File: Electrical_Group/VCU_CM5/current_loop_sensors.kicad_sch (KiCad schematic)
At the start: 16 parts, among them J11 Conn_01x30_Socket

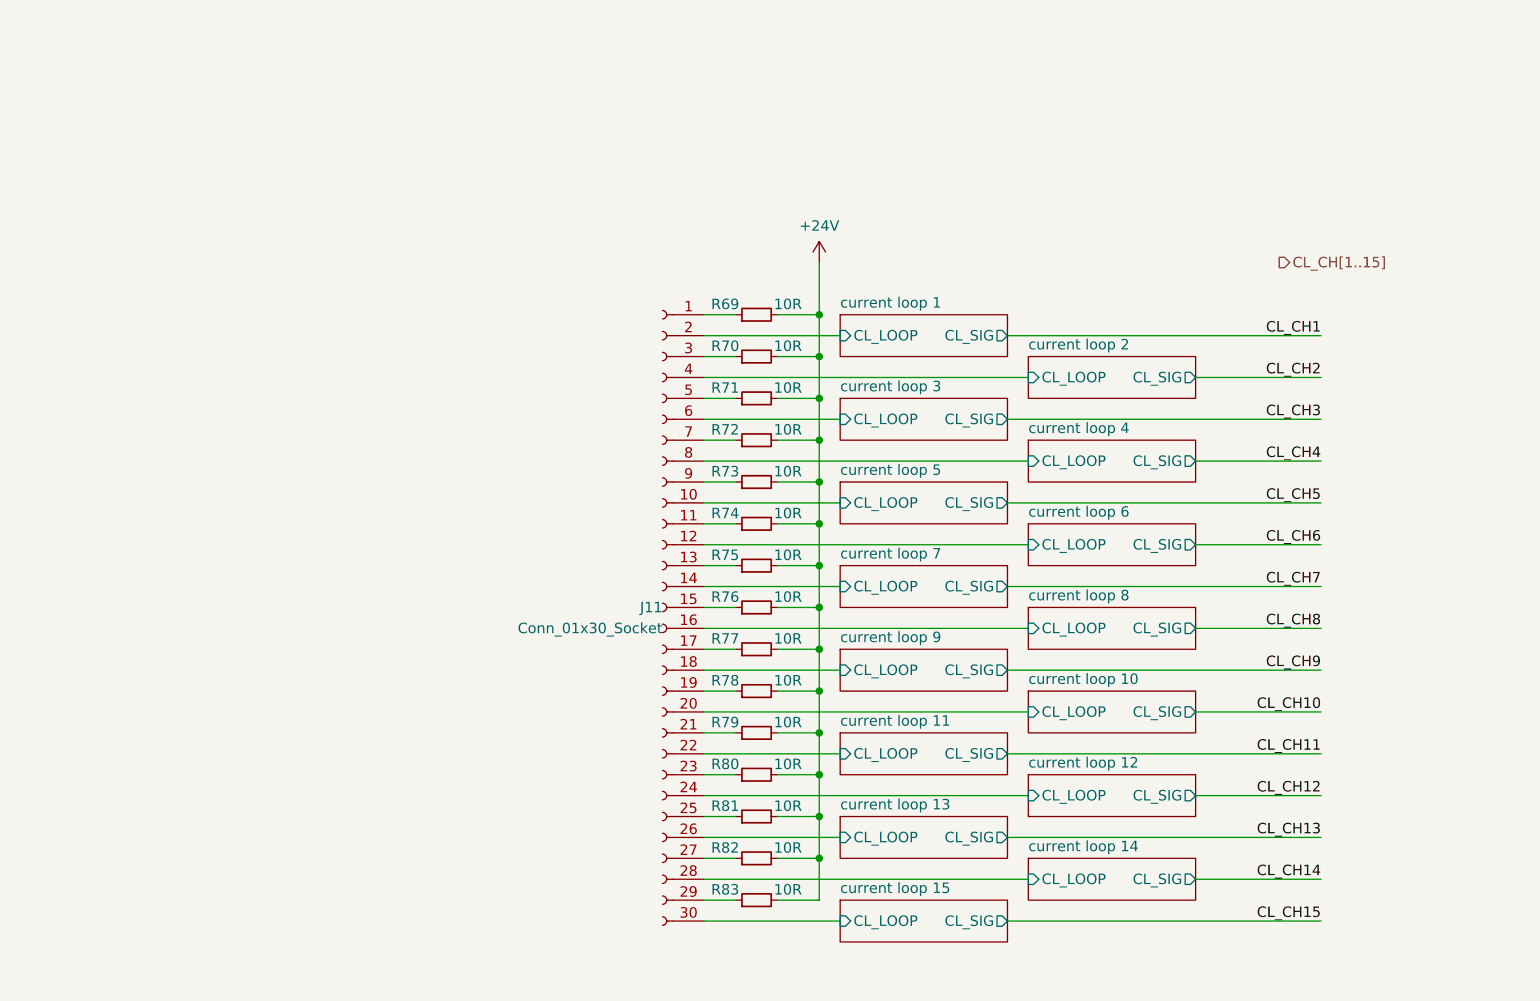
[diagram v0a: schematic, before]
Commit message: [VCU_CM5] update to V1.0
still needs many modifications
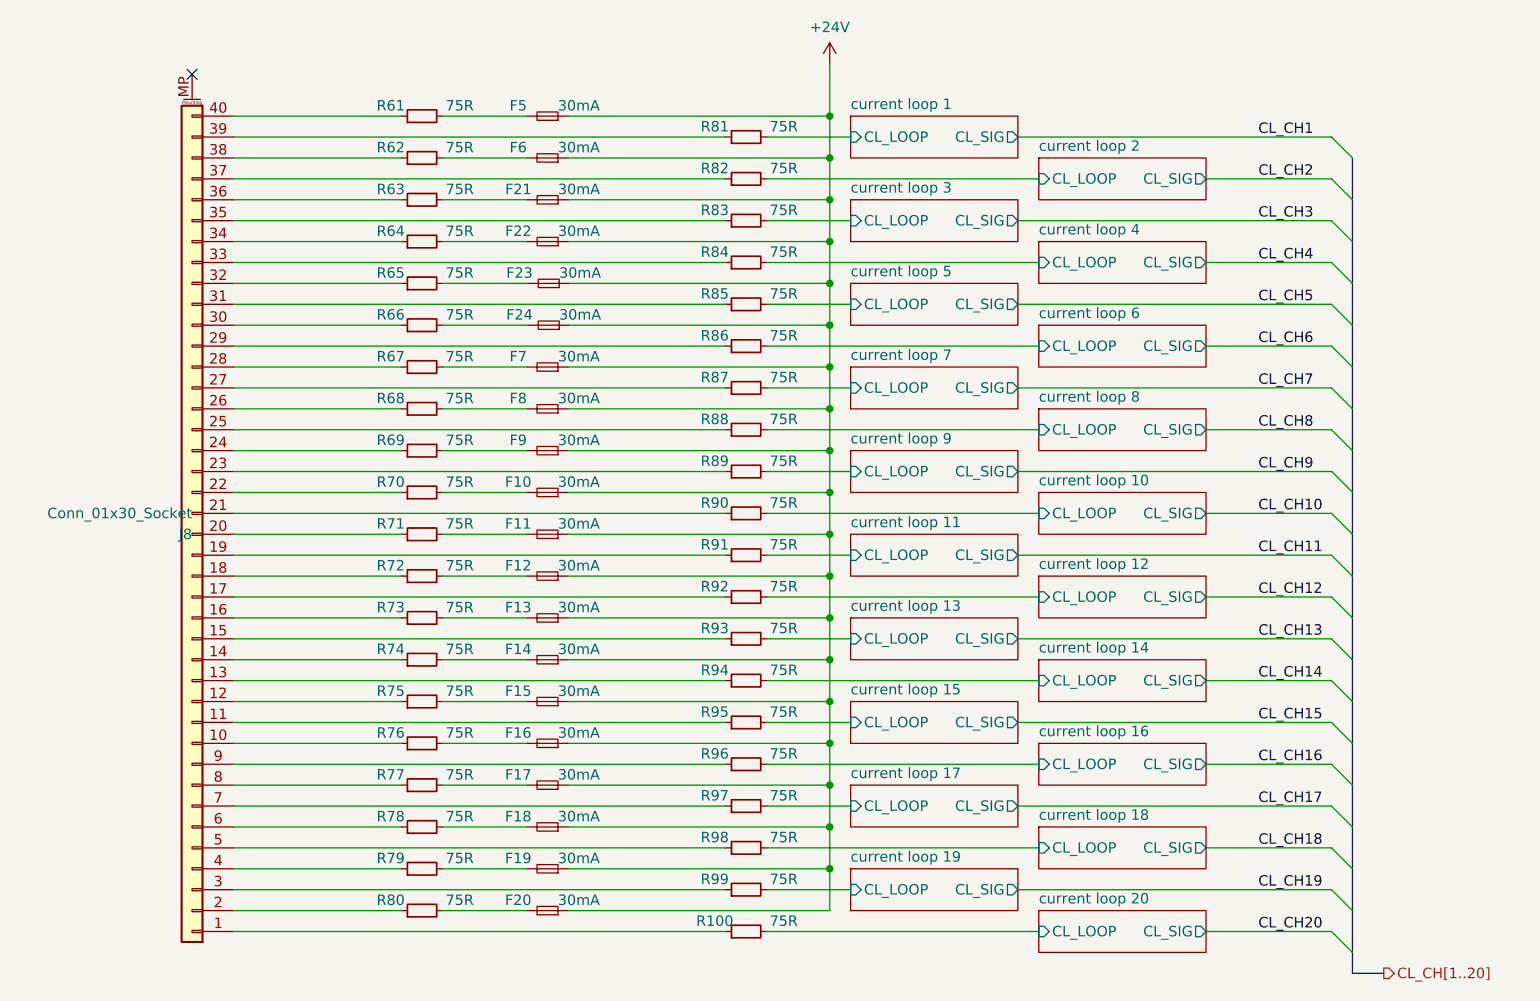
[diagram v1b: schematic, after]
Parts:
- added F10, F11, F12, F13, F14, F15, F16, F17, F18, F19, F20, F21, F22, F23, F24, F5, F6, F7, F8, F9: 30mA, Fuse:Fuse_0805_2012Metric_Pad1.15x1.40mm_HandSolder, symbol Device:Fuse_Small
- added R100, R81, R82, R83, R84, R85, R86, R87, R88, R89, R90, R91, R92, R93, R94, R95, R96, R97, R98, R99: 75R, Resistor_SMD:R_0603_1608Metric, symbol Device:R_Small
- added R76, R77, R78, R79, R80: 75R, Resistor_SMD:R_0603_1608Metric_Pad0.98x0.95mm_HandSolder, symbol Device:R_Small
- J8: renamed from J11; footprint Connector_FFC-FPC:Amphenol_F32Q-1A7x1-11030_1x30-1MP_P0.5mm_Horizontal -> Connector_FFC-FPC:Amphenol_F32Q-1A7x1-11040_1x40-1MP_P0.5mm_Horizontal; symbol Connector:Conn_01x30_Socket -> Connector_Generic_MountingPin:Conn_01x40_MountingPin
- R61: renamed from R69; value 10R -> 75R; footprint Resistor_SMD:R_0603_1608Metric -> Resistor_SMD:R_0603_1608Metric_Pad0.98x0.95mm_HandSolder
- R62: renamed from R70; value 10R -> 75R; footprint Resistor_SMD:R_0603_1608Metric -> Resistor_SMD:R_0603_1608Metric_Pad0.98x0.95mm_HandSolder
- R63: renamed from R71; value 10R -> 75R; footprint Resistor_SMD:R_0603_1608Metric -> Resistor_SMD:R_0603_1608Metric_Pad0.98x0.95mm_HandSolder
- R64: renamed from R72; value 10R -> 75R; footprint Resistor_SMD:R_0603_1608Metric -> Resistor_SMD:R_0603_1608Metric_Pad0.98x0.95mm_HandSolder
- R65: renamed from R73; value 10R -> 75R; footprint Resistor_SMD:R_0603_1608Metric -> Resistor_SMD:R_0603_1608Metric_Pad0.98x0.95mm_HandSolder
- R66: renamed from R74; value 10R -> 75R; footprint Resistor_SMD:R_0603_1608Metric -> Resistor_SMD:R_0603_1608Metric_Pad0.98x0.95mm_HandSolder
- R67: renamed from R75; value 10R -> 75R; footprint Resistor_SMD:R_0603_1608Metric -> Resistor_SMD:R_0603_1608Metric_Pad0.98x0.95mm_HandSolder
- R68: renamed from R76; value 10R -> 75R; footprint Resistor_SMD:R_0603_1608Metric -> Resistor_SMD:R_0603_1608Metric_Pad0.98x0.95mm_HandSolder
- R69: renamed from R77; value 10R -> 75R; footprint Resistor_SMD:R_0603_1608Metric -> Resistor_SMD:R_0603_1608Metric_Pad0.98x0.95mm_HandSolder
- R70: renamed from R78; value 10R -> 75R; footprint Resistor_SMD:R_0603_1608Metric -> Resistor_SMD:R_0603_1608Metric_Pad0.98x0.95mm_HandSolder
- R71: renamed from R79; value 10R -> 75R; footprint Resistor_SMD:R_0603_1608Metric -> Resistor_SMD:R_0603_1608Metric_Pad0.98x0.95mm_HandSolder
- R72: renamed from R80; value 10R -> 75R; footprint Resistor_SMD:R_0603_1608Metric -> Resistor_SMD:R_0603_1608Metric_Pad0.98x0.95mm_HandSolder
- R73: renamed from R81; value 10R -> 75R; footprint Resistor_SMD:R_0603_1608Metric -> Resistor_SMD:R_0603_1608Metric_Pad0.98x0.95mm_HandSolder
- R74: renamed from R82; value 10R -> 75R; footprint Resistor_SMD:R_0603_1608Metric -> Resistor_SMD:R_0603_1608Metric_Pad0.98x0.95mm_HandSolder
- R75: renamed from R83; value 10R -> 75R; footprint Resistor_SMD:R_0603_1608Metric -> Resistor_SMD:R_0603_1608Metric_Pad0.98x0.95mm_HandSolder
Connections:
- net +24V: now also F10.1, F11.1, F12.1, F13.1, F14.1, F15.1, F16.1, F17.1, F18.1, F19.1, F20.1, F21.1, F22.1, F23.1, F24.1, F5.1, F6.1, F7.1, F8.1, F9.1; no longer R61.2, R62.2, R63.2, R64.2, R65.2, R66.2, R67.2, R68.2, R69.2, R70.2, R71.2, R72.2, R73.2, R74.2, R75.2
- net current loop 1/CL_LOOP: now also R81.2; no longer J8.2 (Pin_2)
- net current loop 10/CL_LOOP: now also R90.2; no longer J8.20 (Pin_20)
- net current loop 11/CL_LOOP: now also R91.2; no longer J8.22 (Pin_22)
- net current loop 12/CL_LOOP: now also R92.2; no longer J8.24 (Pin_24)
- net current loop 13/CL_LOOP: now also R93.2; no longer J8.26 (Pin_26)
- net current loop 14/CL_LOOP: now also R94.2; no longer J8.28 (Pin_28)
- net current loop 15/CL_LOOP: now also R95.2; no longer J8.30 (Pin_30)
- net current loop 2/CL_LOOP: now also R82.2; no longer J8.4 (Pin_4)
- net current loop 3/CL_LOOP: now also R83.2; no longer J8.6 (Pin_6)
- net current loop 4/CL_LOOP: now also R84.2; no longer J8.8 (Pin_8)
- net current loop 5/CL_LOOP: now also R85.2; no longer J8.10 (Pin_10)
- net current loop 6/CL_LOOP: now also R86.2; no longer J8.12 (Pin_12)
- net current loop 7/CL_LOOP: now also R87.2; no longer J8.14 (Pin_14)
- net current loop 8/CL_LOOP: now also R88.2; no longer J8.16 (Pin_16)
- net current loop 9/CL_LOOP: now also R89.2; no longer J8.18 (Pin_18)
- net at R71.1: now also J8.20 (Pin_20); no longer J8.21 (Pin_21)
- net at R67.1: now also J8.28 (Pin_28); no longer J8.13 (Pin_13)
- net at R75.1: now also J8.12 (Pin_12); no longer J8.29 (Pin_29)
- net at R68.1: now also J8.26 (Pin_26); no longer J8.15 (Pin_15)
- net at R70.1: now also J8.22 (Pin_22); no longer J8.19 (Pin_19)
- net at R73.1: now also J8.16 (Pin_16); no longer J8.25 (Pin_25)
- net at R65.1: now also J8.32 (Pin_32); no longer J8.9 (Pin_9)
- net at R64.1: now also J8.34 (Pin_34); no longer J8.7 (Pin_7)
- net at J8.3 (Pin_3): now also R99.1; no longer R62.1
- net at R66.1: now also J8.30 (Pin_30); no longer J8.11 (Pin_11)
- net at R74.1: now also J8.14 (Pin_14); no longer J8.27 (Pin_27)
- net at R63.1: now also J8.36 (Pin_36); no longer J8.5 (Pin_5)
- net at J8.1 (Pin_1): now also R100.1; no longer R61.1
- net at J8.17 (Pin_17): now also R92.1; no longer R69.1
- net at J8.23 (Pin_23): now also R89.1; no longer R72.1
- new net: F20.2, R80.2
- new net: F11.2, R71.2
- new net: J8.31 (Pin_31), R85.1
- new net: F7.2, R67.2
- new net: J8.21 (Pin_21), R90.1
- new net: F15.2, R75.2
- new net: F9.2, R69.2
- new net: F8.2, R68.2
- new net: F16.2, R76.2
- new net: J8.6 (Pin_6), R78.1
- new net: F18.2, R78.2
- new net: F6.2, R62.2
- new net: F10.2, R70.2
- new net: F13.2, R73.2
- new net: J8.8 (Pin_8), R77.1
- new net: F17.2, R77.2
- new net: F24.2, R66.2
- new net: F23.2, R65.2
- new net: F19.2, R79.2
- new net: J8.35 (Pin_35), R83.1
- new net: J8.33 (Pin_33), R84.1
- new net: F12.2, R72.2
- new net: J8.13 (Pin_13), R94.1
- new net: F22.2, R64.2
- new net: J8.39 (Pin_39), R81.1
- new net: J8.38 (Pin_38), R62.1
- new net: F14.2, R74.2
- new net: F5.2, R61.2
- new net: J8.25 (Pin_25), R88.1
- new net: F21.2, R63.2
- new net: J8.10 (Pin_10), R76.1
- new net: J8.11 (Pin_11), R95.1
- new net: J8.15 (Pin_15), R93.1
- new net: J8.18 (Pin_18), R72.1
- new net: J8.19 (Pin_19), R91.1
- new net: J8.2 (Pin_2), R80.1
- new net: J8.24 (Pin_24), R69.1
- new net: J8.27 (Pin_27), R87.1
- new net: J8.29 (Pin_29), R86.1
- new net: J8.37 (Pin_37), R82.1
- new net: J8.4 (Pin_4), R79.1
- new net: J8.40 (Pin_40), R61.1
- new net: J8.5 (Pin_5), R98.1
- new net: J8.7 (Pin_7), R97.1
- new net: J8.9 (Pin_9), R96.1
- new net current loop 16/CL_LOOP: R96.2
- new net current loop 17/CL_LOOP: R97.2
- new net current loop 18/CL_LOOP: R98.2
- new net current loop 19/CL_LOOP: R99.2
- new net current loop 20/CL_LOOP: R100.2
- no-connect marks 0 -> 1
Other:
- added sheet current loop 16 (current loop.kicad_sch)
- added sheet current loop 17 (current loop.kicad_sch)
- added sheet current loop 18 (current loop.kicad_sch)
- added sheet current loop 19 (current loop.kicad_sch)
- added sheet current loop 20 (current loop.kicad_sch)
- company: (none) -> NTURacing Team
- title: (none) -> VCU_CM5
- moved on the sheet: R61, R62, R63, R64, R65, R66, R67, R68, R69, R70, R71, R72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
